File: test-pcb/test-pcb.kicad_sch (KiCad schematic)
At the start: 17 parts, among them IC1 VNH5019ATR-E, J1 Conn_01x06, J2 Conn_01x06, J3 Conn_01x03, Q1 IPD050N10N5ATMA1

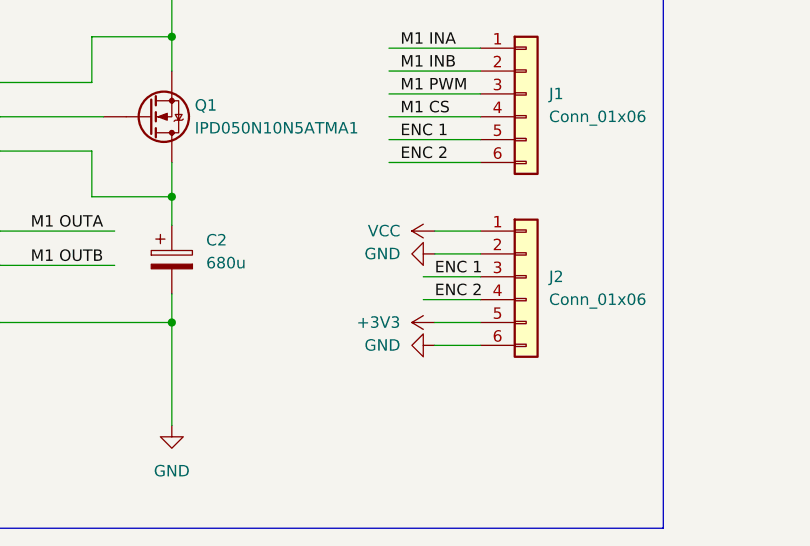
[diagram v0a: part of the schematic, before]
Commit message: test - fixed mdriver sch
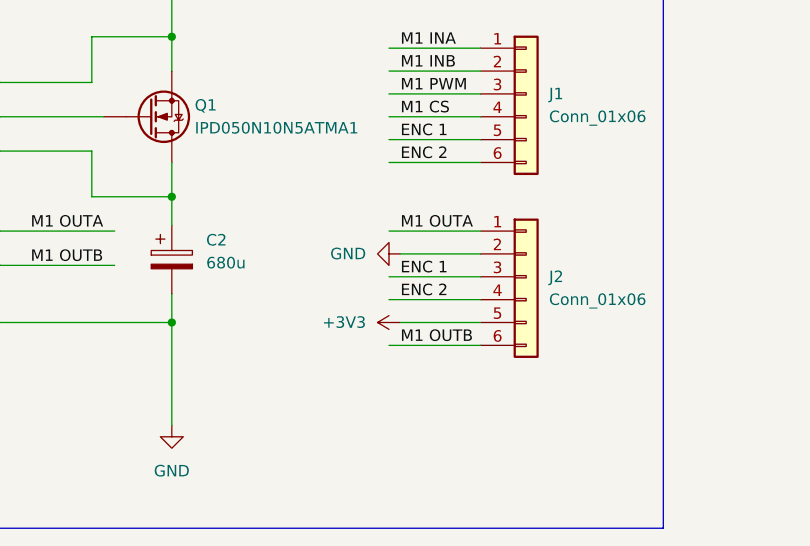
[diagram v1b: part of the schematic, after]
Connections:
- net GND: no longer J2.6 (Pin_6)
- net M1 OUTA: now also J2.1 (Pin_1)
- net M1 OUTB: now also J2.6 (Pin_6)
- net VCC: no longer J2.1 (Pin_1)
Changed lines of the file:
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@@
   (junction (at 101.6 39.37) (diameter 0) (color 0 0 0 0)
   )
-  (wire (pts (xy 130.81 73.66) (xy 135.89 73.66))
+  (wire (pts (xy 125.73 73.66) (xy 135.89 73.66))
     (stroke (width 0) (type default))
   )
@@
     (stroke (width 0) (type default))
   )
-  (wire (pts (xy 130.81 63.5) (xy 135.89 63.5))
-    (stroke (width 0) (type default))
-  )
   (wire (pts (xy 101.6 26.67) (xy 101.6 39.37))
     (stroke (width 0) (type default))
@@
     (stroke (width 0) (type default))
   )
-  (wire (pts (xy 129.54 66.04) (xy 135.89 66.04))
-    (stroke (width 0) (type default))
-  )
-  (wire (pts (xy 129.54 68.58) (xy 135.89 68.58))
+  (wire (pts (xy 125.73 66.04) (xy 135.89 66.04))
+    (stroke (width 0) (type default))
+  )
+  (wire (pts (xy 125.73 68.58) (xy 135.89 68.58))
     (stroke (width 0) (type default))
   )
@@
     (stroke (width 0) (type default))
   )
+  (wire (pts (xy 127 63.5) (xy 135.89 63.5))
+    (stroke (width 0) (type default))
+  )
   (wire (pts (xy 25.4 44.45) (xy 31.75 44.45))
     (stroke (width 0) (type default))
@@
     (stroke (width 0) (type default))
   )
-  (wire (pts (xy 130.81 60.96) (xy 135.89 60.96))
+  (wire (pts (xy 125.73 60.96) (xy 135.89 60.96))
     (stroke (width 0) (type default))
   )
@@
     (stroke (width 0) (type default))
   )
-  (wire (pts (xy 130.81 71.12) (xy 135.89 71.12))
+  (wire (pts (xy 127 71.12) (xy 135.89 71.12))
     (stroke (width 0) (type default))
   )
@@
     (effects (font (size 1.27 1.27)) (justify right bottom))
   )
-  (label "ENC 1" (at 130.81 66.04 0) (fields_autoplaced)
+  (label "ENC 1" (at 127 66.04 0) (fields_autoplaced)
     (effects (font (size 1.27 1.27)) (justify left bottom))
   )
@@
     (effects (font (size 1.27 1.27)) (justify left bottom))
   )
-  (label "ENC 2" (at 130.81 68.58 0) (fields_autoplaced)
+  (label "ENC 2" (at 127 68.58 0) (fields_autoplaced)
     (effects (font (size 1.27 1.27)) (justify left bottom))
   )
@@
     (effects (font (size 1.27 1.27)) (justify left bottom))
   )
+  (label "M1 OUTA" (at 127 60.96 0) (fields_autoplaced)
+    (effects (font (size 1.27 1.27)) (justify left bottom))
+  )
   (label "M1 PWM" (at 26.67 62.23 0) (fields_autoplaced)
     (effects (font (size 1.27 1.27)) (justify left bottom))
   )
   (label "ENC 2" (at 127 53.34 0) (fields_autoplaced)
+    (effects (font (size 1.27 1.27)) (justify left bottom))
+  )
+  (label "M1 OUTB" (at 127 73.66 0) (fields_autoplaced)
     (effects (font (size 1.27 1.27)) (justify left bottom))
   )
@@
     )
   )
-  (symbol (lib_id "power:GND") (at 130.81 63.5 270) (mirror x) (unit 1)
-    (in_bom yes) (on_board yes) (dnp no) (fields_autoplaced)
-    (property "Reference" "#PWR013" (at 124.46 63.5 0)
-      (effects (font (size 1.27 1.27)) hide)
-    )
-    (property "Value" "GND" (at 127 63.4999 90)
+  (symbol (lib_id "power:GND") (at 127 63.5 270) (mirror x) (unit 1)
+    (in_bom yes) (on_board yes) (dnp no) (fields_autoplaced)
+    (property "Reference" "#PWR013" (at 120.65 63.5 0)
+      (effects (font (size 1.27 1.27)) hide)
+    )
+    (property "Value" "GND" (at 123.19 63.4999 90)
       (effects (font (size 1.27 1.27)) (justify right))
     )
-    (property "Footprint" "" (at 130.81 63.5 0)
-      (effects (font (size 1.27 1.27)) hide)
-    )
-    (property "Datasheet" "" (at 130.81 63.5 0)
+    (property "Footprint" "" (at 127 63.5 0)
+      (effects (font (size 1.27 1.27)) hide)
+    )
+    (property "Datasheet" "" (at 127 63.5 0)
       (effects (font (size 1.27 1.27)) hide)
     )
@@
     )
   )
-  (symbol (lib_id "power:+3V3") (at 130.81 71.12 90) (mirror x) (unit 1)
-    (in_bom yes) (on_board yes) (dnp no) (fields_autoplaced)
-    (property "Reference" "#PWR011" (at 134.62 71.12 0)
-      (effects (font (size 1.27 1.27)) hide)
-    )
-    (property "Value" "+3V3" (at 127 71.1201 90)
-      (effects (font (size 1.27 1.27)) (justify left))
-    )
-    (property "Footprint" "" (at 130.81 71.12 0)
-      (effects (font (size 1.27 1.27)) hide)
-    )
-    (property "Datasheet" "" (at 130.81 71.12 0)
+  (symbol (lib_id "power:+3V3") (at 127 71.12 90) (mirror x) (unit 1)
+    (in_bom yes) (on_board yes) (dnp no) (fields_autoplaced)
+    (property "Reference" "#PWR011" (at 130.81 71.12 0)
+      (effects (font (size 1.27 1.27)) hide)
+    )
+    (property "Value" "+3V3" (at 123.19 71.1201 90)
+      (effects (font (size 1.27 1.27)) (justify left))
+    )
+    (property "Footprint" "" (at 127 71.12 0)
+      (effects (font (size 1.27 1.27)) hide)
+    )
+    (property "Datasheet" "" (at 127 71.12 0)
       (effects (font (size 1.27 1.27)) hide)
     )
@@
     )
   )
-  (symbol (lib_id "power:VCC") (at 130.81 60.96 90) (mirror x) (unit 1)
-    (in_bom yes) (on_board yes) (dnp no) (fields_autoplaced)
-    (property "Reference" "#PWR09" (at 134.62 60.96 0)
-      (effects (font (size 1.27 1.27)) hide)
-    )
-    (property "Value" "VCC" (at 127 60.9599 90)
-      (effects (font (size 1.27 1.27)) (justify left))
-    )
-    (property "Footprint" "" (at 130.81 60.96 0)
-      (effects (font (size 1.27 1.27)) hide)
-    )
-    (property "Datasheet" "" (at 130.81 60.96 0)
-      (effects (font (size 1.27 1.27)) hide)
-    )
-    (pin "1")
-    (instances
-      (project "test-pcb"
-        (path "/1cd04cc7-ac63-4801-a234-4389545ae7cf"
-          (reference "#PWR09") (unit 1)
-        )
-      )
-    )
-  )
   (symbol (lib_id "power:GND") (at 101.6 82.55 0) (unit 1)
     (in_bom yes) (on_board yes) (dnp no) (fields_autoplaced)
@@
         )
       )
-    )
-  )
-  (symbol (lib_id "power:GND") (at 130.81 73.66 270) (mirror x) (unit 1)
-    (in_bom yes) (on_board yes) (dnp no) (fields_autoplaced)
-    (property "Reference" "#PWR010" (at 124.46 73.66 0)
-      (effects (font (size 1.27 1.27)) hide)
-    )
-    (property "Value" "GND" (at 127 73.6599 90)
-      (effects (font (size 1.27 1.27)) (justify right))
-    )
-    (property "Footprint" "" (at 130.81 73.66 0)
-      (effects (font (size 1.27 1.27)) hide)
-    )
-    (property "Datasheet" "" (at 130.81 73.66 0)
-      (effects (font (size 1.27 1.27)) hide)
-    )
-    (pin "1")
-    (instances
-      (project "test-pcb"
-        (path "/1cd04cc7-ac63-4801-a234-4389545ae7cf"
-          (reference "#PWR010") (unit 1)
-        )
-      )
